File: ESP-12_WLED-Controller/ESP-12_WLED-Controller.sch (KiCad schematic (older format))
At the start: 21 parts, among them J1 Conn_01x02_Male, J2 Conn_01x04_Male, J3 Conn_01x03_Male, Q1 BC847, Q2 IRF7404, SW1 SW_RST, U1 TS1117-3.3, U2 ESP-12E, U3 SN74LVC1T45DBV

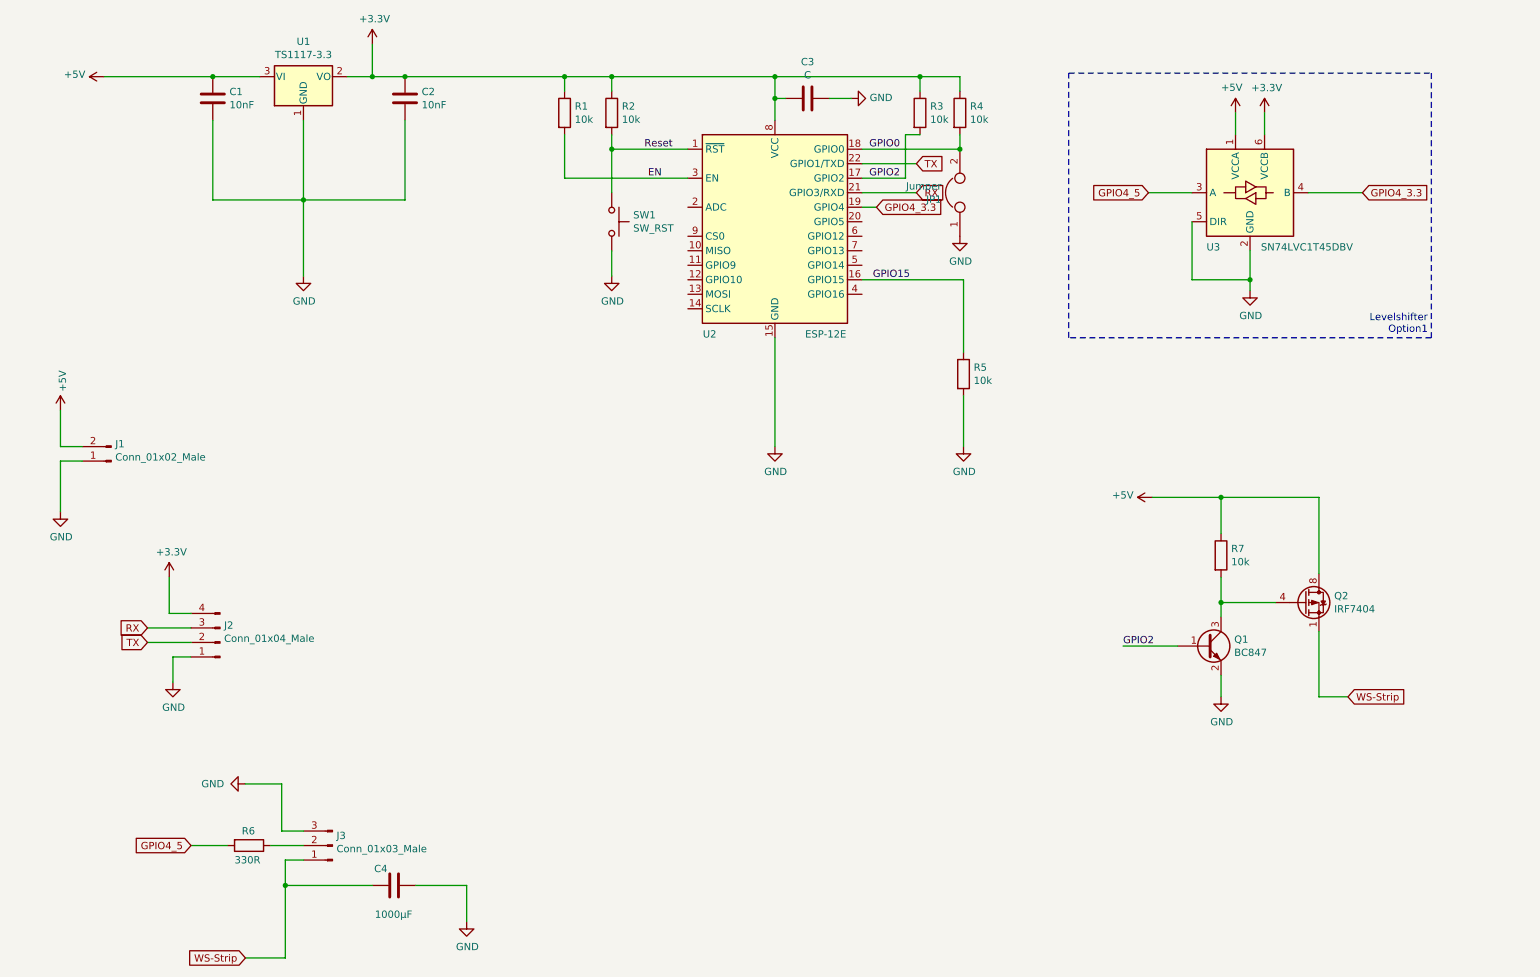
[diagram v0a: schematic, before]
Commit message: LLC changes
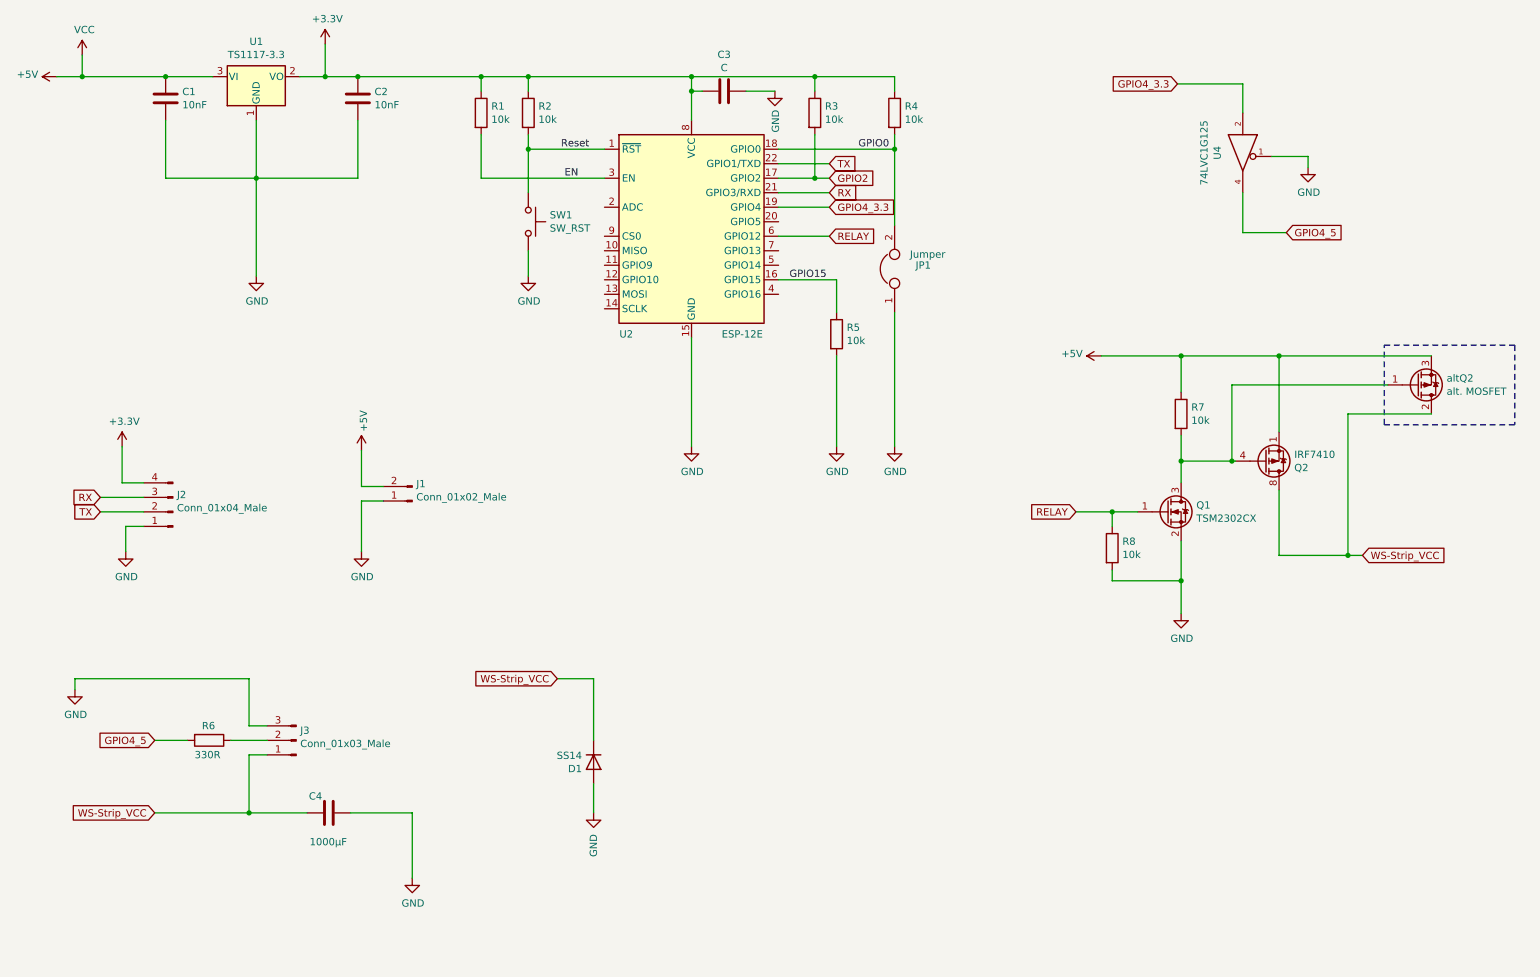
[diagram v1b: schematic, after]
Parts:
- removed Q1: BC847, Package_TO_SOT_SMD:SOT-23, symbol Transistor_BJT:BC847
- removed U3: SN74LVC1T45DBV, Package_TO_SOT_SMD:SOT-23-6, symbol Logic_LevelTranslator:SN74LVC1T45DBV
- added D1: SS14, Diode_SMD:D_SMA_Handsoldering, symbol Device:D
- added Q1: TSM2302CX, Package_TO_SOT_SMD:SOT-23, symbol Transistor_FET:TSM2302CX
- added R8: 10k, Resistor_SMD:R_0805_2012Metric_Pad1.15x1.40mm_HandSolder, symbol Device:R
- added U4: 74LVC1G125, Package_SO:TSOP-5_1.65x3.05mm_P0.95mm, symbol 74xGxx:74LVC1G125
- added altQ2: alt. MOSFET, Package_TO_SOT_THT:TO-220-3_Vertical, symbol Transistor_FET:IRF9540N
- Q2: value IRF7404 -> IRF7410
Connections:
- net +5V: now also Q2.1 (S), Q2.2 (S), Q2.3 (S), U4.5 (VCC), altQ2.3 (S); no longer Q2.5 (D), Q2.6 (D), Q2.7 (D), Q2.8 (D)
- net GND: now also D1.2 (A), Q1.2 (S), R8.2, U4.1, U4.3 (GND)
- net GPIO4_3.3: now also U4.2
- net GPIO4_5: now also U4.4
- net RELAY: now reaches U2.6 (GPIO12)
- net RELAY: now also Q1.1 (G), R8.1
- net at Q2.4 (G), R7.2: now also Q1.3 (D), altQ2.1 (G)
- removed net WS-Strip: C4.1, J3.1 (Pin_1), Q2.1 (S), Q2.2 (S), Q2.3 (S)
- new net WS-Strip_VCC: C4.1, D1.1 (K), J3.1 (Pin_1), Q2.5 (D), Q2.6 (D), Q2.7 (D), Q2.8 (D), altQ2.2 (D)
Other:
- note removed: "Levelshifter\nOption1"
- moved on the sheet: C1, C2, C3, C4, J1, J2, J3, JP1, Q2, R1, R2, R3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
